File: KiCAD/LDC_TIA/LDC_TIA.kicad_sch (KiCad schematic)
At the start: 19 parts, among them J1 Conn_01x02_Pin, J2 Conn_01x06_Pin, J3 54-00166, Q1 BC817, SW1 SW_SPST, U1 OPA2197xDGK, U2 LM7805_TO220

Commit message: Initial Commit
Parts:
- J3: footprint JACK:TENSILITY_54-00166 -> Footprints:TENSILITY_54-00166
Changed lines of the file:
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@@
 			)
 		)
-		(property "Footprint" "JACK:TENSILITY_54-00166"
+		(property "Footprint" "Footprints:TENSILITY_54-00166"
 			(at 91.44 107.95 0)
 			(effects

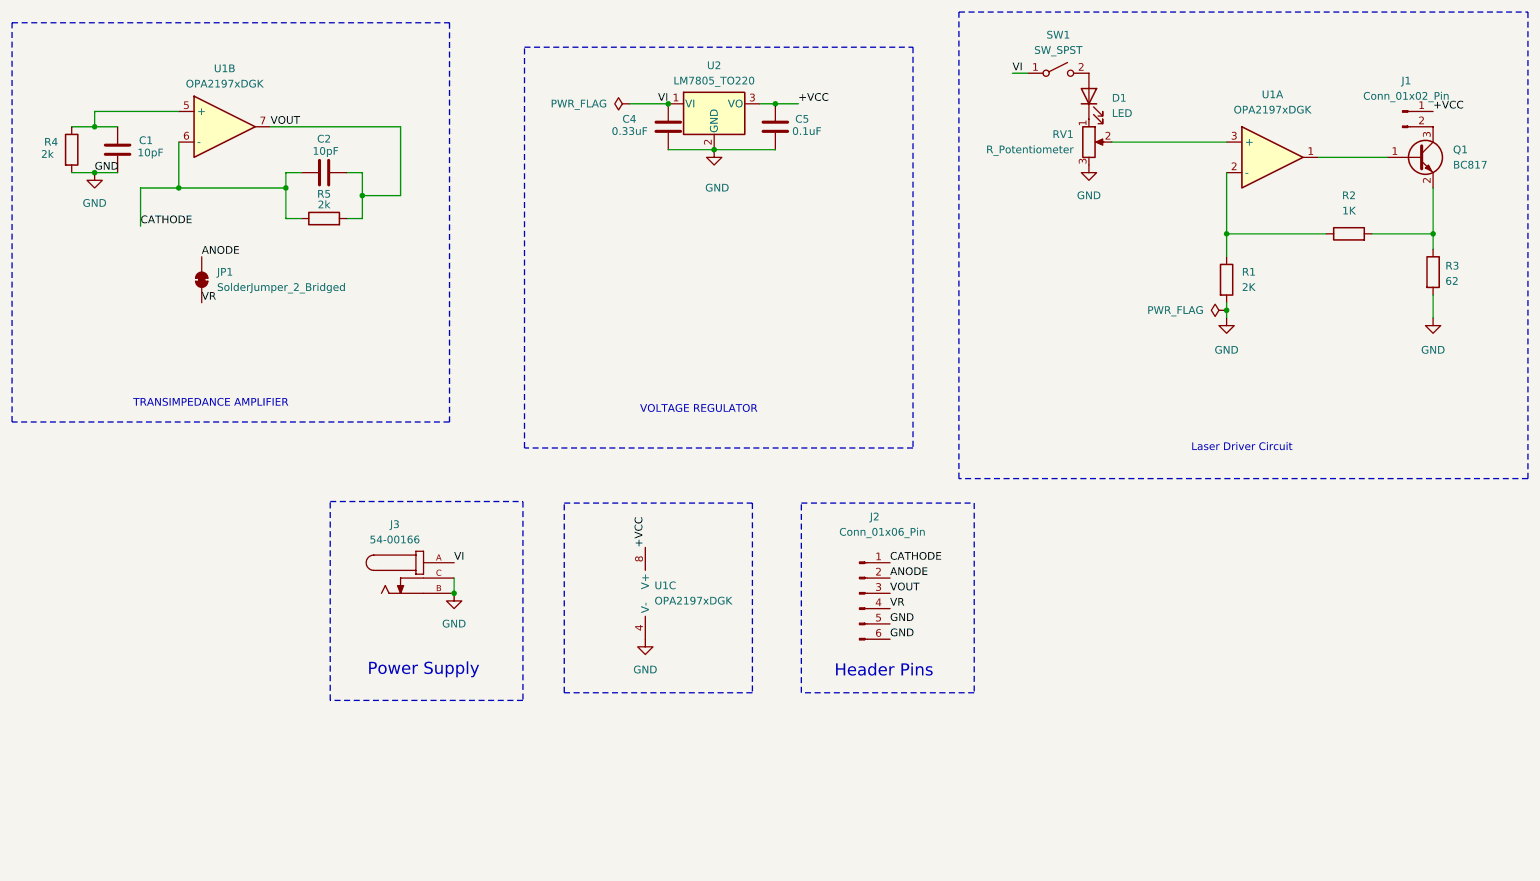
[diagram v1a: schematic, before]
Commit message: Done with Schematics V1
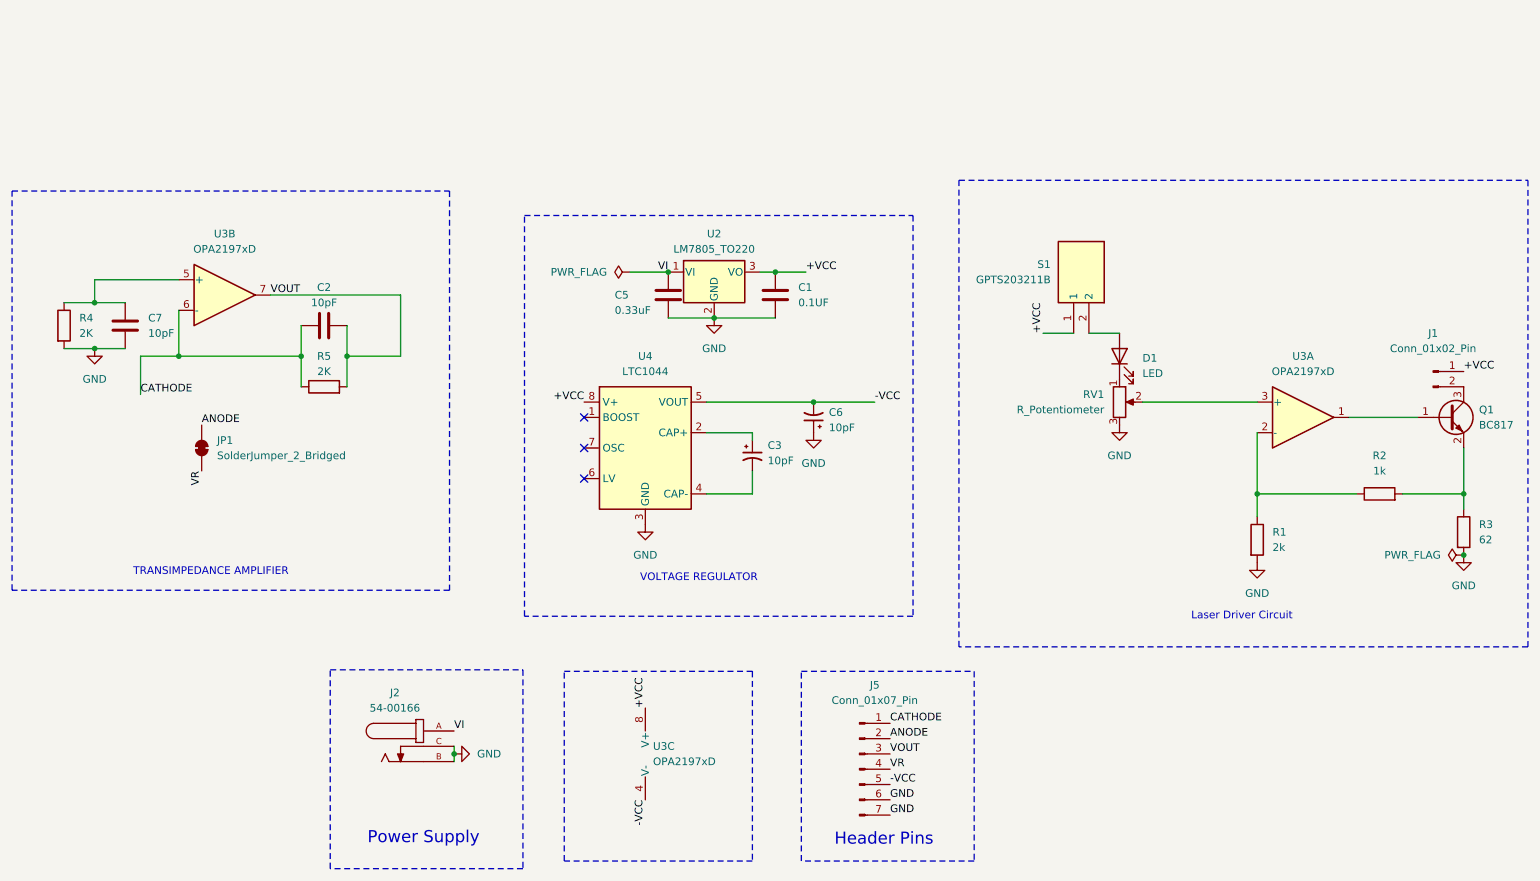
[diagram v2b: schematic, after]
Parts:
- removed C1, C2: 10pF, Capacitor_SMD:C_0201_0603Metric, symbol Library:C
- removed C4: 0.33uF, Capacitor_SMD:C_0201_0603Metric, symbol Library:C
- removed C5: 0.1uF, Capacitor_SMD:C_0201_0603Metric, symbol Library:C
- removed J2: Conn_01x06_Pin, Connector_PinHeader_2.54mm:PinHeader_1x06_P2.54mm_Vertical, symbol Connector:Conn_01x06_Pin
- removed J3: 54-00166, Footprints:TENSILITY_54-00166, symbol Library:54-00166
- removed Q1: BC817, Package_TO_SOT_SMD:SOT-23, symbol Library:BC817
- removed R1: 2K, Resistor_THT:R_Axial_DIN0207_L6.3mm_D2.5mm_P7.62mm_Horizontal, symbol Library:R
- removed R2: 1K, Resistor_THT:R_Axial_DIN0207_L6.3mm_D2.5mm_P7.62mm_Horizontal, symbol Library:R
- removed R3: 62, Resistor_THT:R_Axial_DIN0309_L9.0mm_D3.2mm_P25.40mm_Horizontal, symbol Library:R
- removed R4, R5: 2k, Resistor_THT:R_Axial_DIN0204_L3.6mm_D1.6mm_P5.08mm_Horizontal, symbol Library:R
- removed SW1: SW_SPST, symbol Switch:SW_SPST
- removed U1: OPA2197xDGK, Package_SO:VSSOP-8_3x3mm_P0.65mm, symbol Library:OPA2197xDGK
- added C1: 0.1UF, FOOTPRINTS:CAP_UEP_5X11_NCH, symbol Device:C
- added C2, C7: 10pF, FOOTPRINTS:CAPRB250W50L400T250H550, symbol Device:C
- added C3, C6: 10pF, FOOTPRINTS:CAPRB250W50L400T250H550, symbol Device:C_Polarized_Small_US
- added C5: 0.33uF, FOOTPRINTS:CAP_UEP_5X11_NCH, symbol Device:C
- added J2: 54-00166, FOOTPRINTS:TENSILITY_54-00166, symbol 54-00166:54-00166
- added J5: Conn_01x07_Pin, Connector_PinHeader_2.54mm:PinHeader_1x07_P2.54mm_Vertical, symbol Connector:Conn_01x07_Pin
- added Q1: BC817, Package_TO_SOT_SMD:SOT-23, symbol potentiometer:BC817
- added R1: 2k, Resistor_THT:R_Axial_DIN0207_L6.3mm_D2.5mm_P7.62mm_Horizontal, symbol Device:R
- added R2: 1k, Resistor_THT:R_Axial_DIN0207_L6.3mm_D2.5mm_P7.62mm_Horizontal, symbol Device:R
- added R3: 62, Resistor_THT:R_Axial_DIN0309_L9.0mm_D3.2mm_P12.70mm_Horizontal, symbol Device:R
- added R4: 2K, Resistor_THT:R_Axial_DIN0207_L6.3mm_D2.5mm_P7.62mm_Horizontal, symbol potentiometer:R
- added R5: 2K, Resistor_THT:R_Axial_DIN0207_L6.3mm_D2.5mm_P7.62mm_Horizontal, symbol Device:R
- added S1: GPTS203211B, FOOTPRINTS:GPTS203211B, symbol GPTS203211B:GPTS203211B
- added U3: OPA2197xD, Package_SO:SOIC-8_3.9x4.9mm_P1.27mm, symbol Amplifier_Operational:OPA2197xD
- added U4: LTC1044, FOOTPRINTS:PDIP-8_N_LIT, symbol Regulator_SwitchedCapacitor:LTC1044
- RV1: footprint (none) -> FOOTPRINTS:potentiometer
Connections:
- net +VCC: now also C1.1, S1.1, U3.8 (V+), U4.8 (V+)
- net ANODE: now also J5.2 (Pin_2)
- net CATHODE: now also C2.1, J5.1 (Pin_1), R5.1, U3.6 (-)
- net GND: now also C1.2, C5.2, C6.1, C7.2, J2.B, J2.C, J5.6 (Pin_6), J5.7 (Pin_7), R1.2, R3.2, R4.2, U4.3 (GND)
- net VI: now also C5.1, J2.A
- net VOUT: now also C2.2, J5.3 (Pin_3), R5.2, U3.7
- net VR: now also J5.4 (Pin_4)
- net at D1.2 (A): now also S1.2
- net at J1.2 (Pin_2): now also Q1.3 (C)
- net at RV1.2: now also U3.3 (+)
- new net: Q1.2 (E), R2.2, R3.1
- new net: C7.1, R4.1, U3.5 (+)
- new net: Q1.1 (B), U3.1
- new net: C3.1, U4.2 (CAP+)
- new net: C3.2, U4.4 (CAP-)
- new net: R1.1, R2.1, U3.2 (-)
- new net -VCC: C6.2, J5.5 (Pin_5), U3.4 (V-), U4.5 (VOUT)
- no-connect marks 0 -> 3
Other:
- moved on the sheet: D1, J1, JP1, RV1, U2
